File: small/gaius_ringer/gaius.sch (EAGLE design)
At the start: 30 parts, among them Q1 2N5088, Q2 2N3906, Q3 2N5088

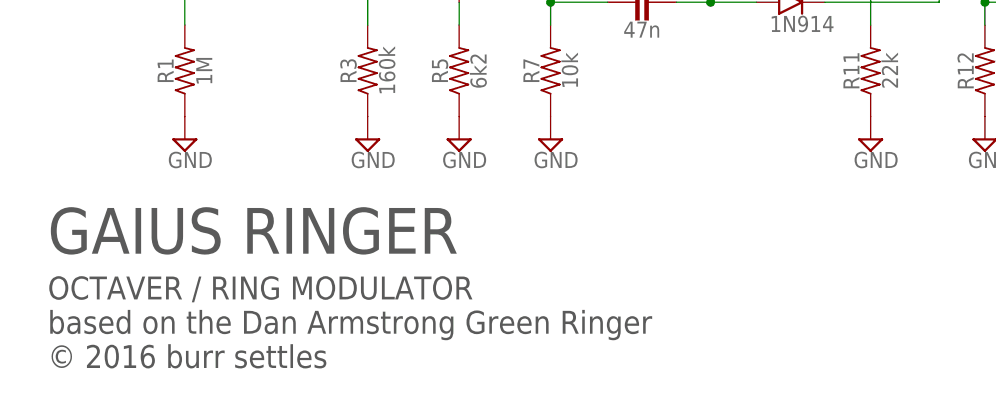
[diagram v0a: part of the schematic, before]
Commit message: formatting updates
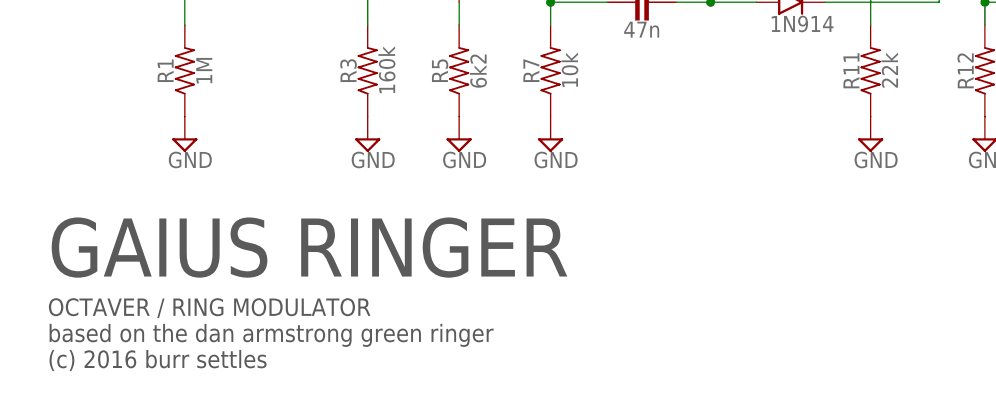
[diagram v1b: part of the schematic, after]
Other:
- note added: "OCTAVER / RING MODULATOR based on the dan armstrong green ringer (c) 2016 burr settles"
- note removed: "OCTAVER / RING MODULATOR based on the Dan Armstrong Green Ringer © 2016 burr settles"
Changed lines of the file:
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@@
 <sheet>
 <plain>
-<text x="2.54" y="15.24" size="5.08" layer="97">GAIUS RINGER</text>
-<text x="2.54" y="2.54" size="2.54" layer="97">OCTAVER / RING MODULATOR
-based on the Dan Armstrong Green Ringer
-© 2016 burr settles</text>
+<text x="2.54" y="12.7" size="6.4516" layer="97">GAIUS RINGER</text>
+<text x="2.54" y="2.54" size="1.9304" layer="97">OCTAVER / RING MODULATOR
+based on the dan armstrong green ringer
+(c) 2016 burr settles</text>
 </plain>
 <instances>
